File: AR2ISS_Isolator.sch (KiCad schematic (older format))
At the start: 21 parts, among them J1 PTT_IN, J12 Conn_01x04, J2 Conn_01x04, J3 Conn_01x04, K1 G6S-2, K2 G6S-2, SW1 SW_Push_SPDT

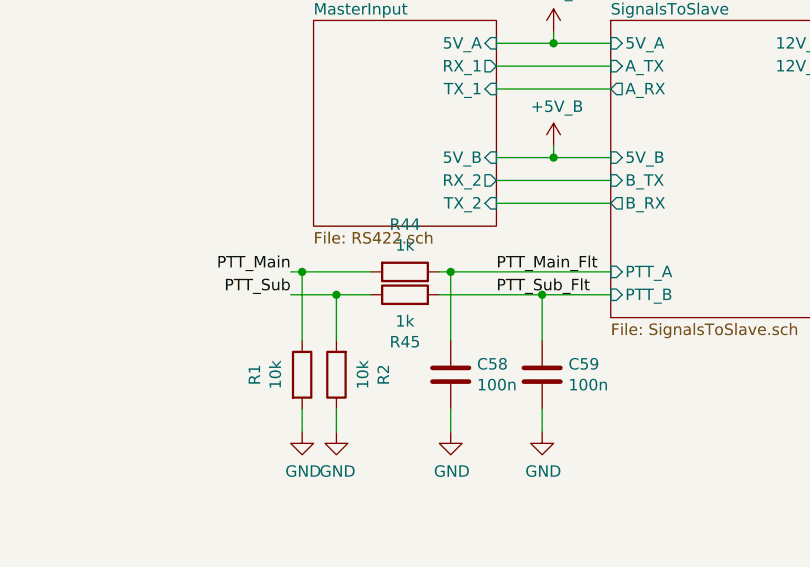
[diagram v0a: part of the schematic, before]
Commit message: added filters
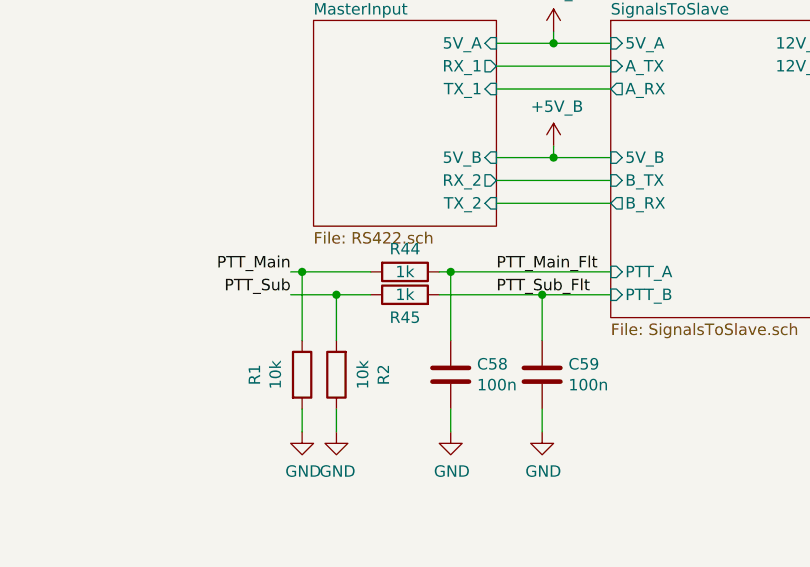
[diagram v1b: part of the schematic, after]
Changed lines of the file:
@@
 $Descr A4 11693 8268
 encoding utf-8
-Sheet 1 19
+Sheet 1 31
 Title ""
 Date ""
@@
 AR Path="/6083EA55/608DE7E0/607F3B85" Ref="R?"  Part="1"
 AR Path="/607F3B85" Ref="R44"  Part="1"
-F 0 "R44" V 5543 3300 50  0000 C CNN
-F 1 "1k" V 5634 3300 50  0000 C CNN
+F 0 "R44" V 5650 3300 50  0000 C CNN
+F 1 "1k" V 5750 3300 50  0000 C CNN
 F 2 "Resistor_SMD:R_0603_1608Metric" V 5680 3300 50  0001 C CNN
 F 3 "~" H 5750 3300 50  0001 C CNN
@@
 AR Path="/6083EA55/608DE7E0/607F46E2" Ref="R?"  Part="1"
 AR Path="/607F46E2" Ref="R45"  Part="1"
-F 0 "R45" V 5543 3400 50  0000 C CNN
-F 1 "1k" V 5634 3400 50  0000 C CNN
+F 0 "R45" V 5650 3400 50  0000 C CNN
+F 1 "1k" V 5750 3400 50  0000 C CNN
 F 2 "Resistor_SMD:R_0603_1608Metric" V 5680 3400 50  0001 C CNN
 F 3 "~" H 5750 3400 50  0001 C CNN
